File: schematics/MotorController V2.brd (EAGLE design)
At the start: 120.6 x 100 mm, 40 parts, among them IC1 7805, Q1 BC307

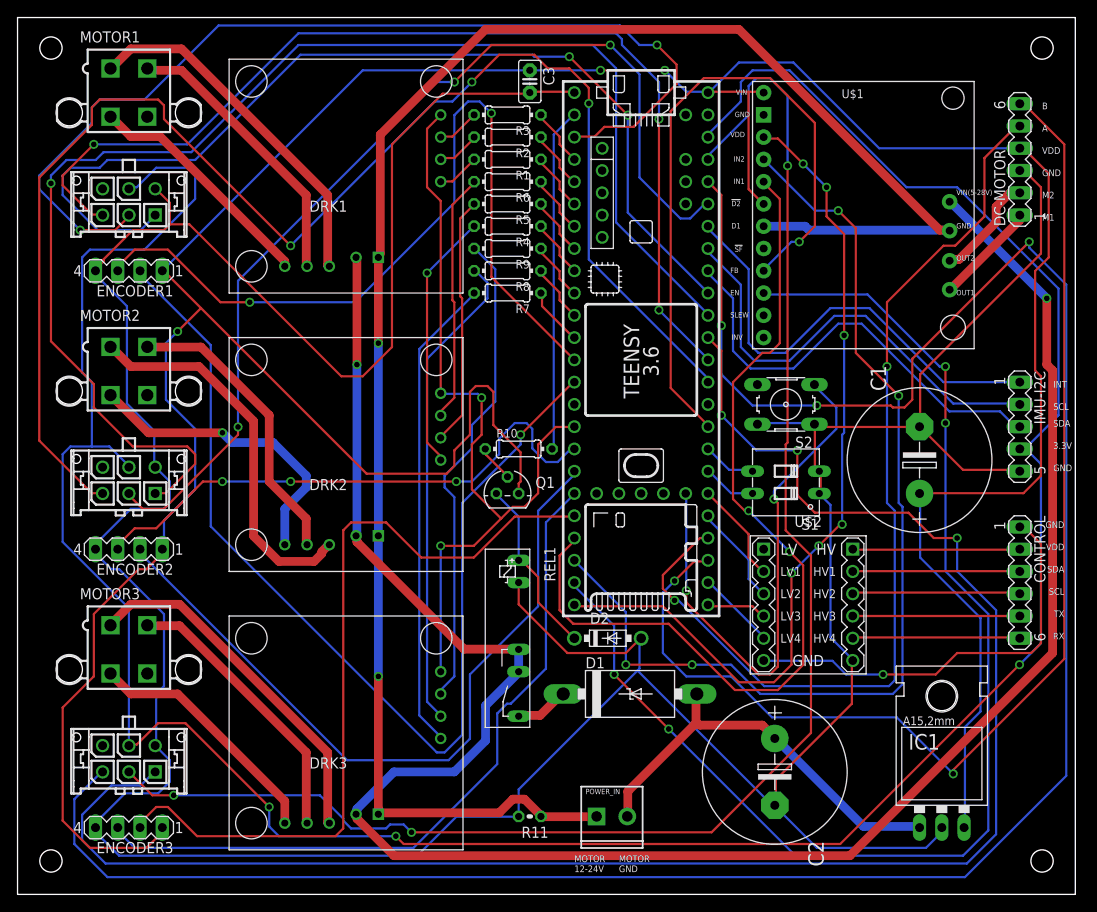
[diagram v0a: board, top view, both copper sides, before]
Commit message: AfterWeekend
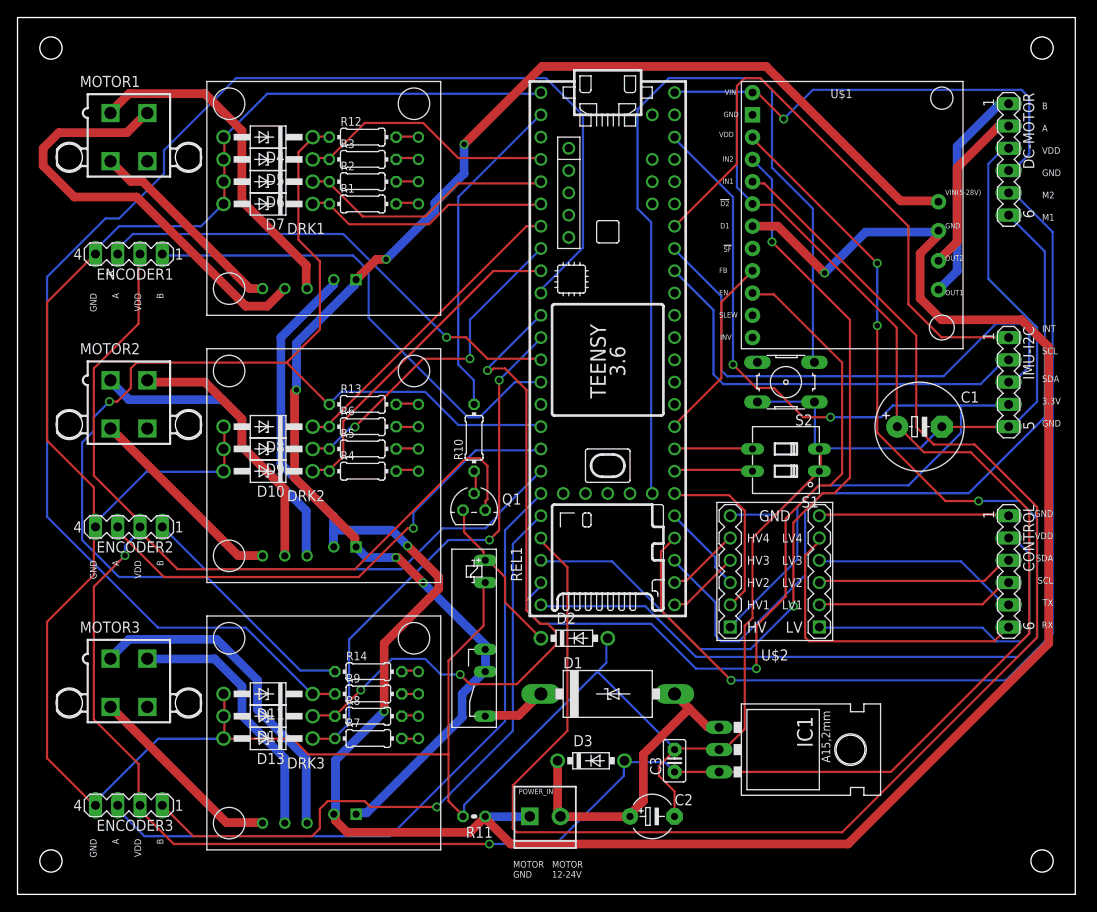
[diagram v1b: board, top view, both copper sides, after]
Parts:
- removed HALL1, HALL2, HALL3: (no value), con-molex-micro-fit-3_0:43045-0612
- added D10, D11, D12, D13, D4, D5, D6, D7, D8, D9: 5.1V, diode:DO41Z10
- added D3: 1N5818-B, diode:DO41-7.6
- added R12, R13, R14: 1K, resistor:0204/7
- C1: value 2200uF -> 1000uF; device rcl:E7,5-16 -> rcl:E5-10,5
- C2: value 2200uF -> 100uF; device rcl:E7,5-16 -> rcl:E5-5
- CONTROL, S1, S2: value (none) -> (none)
- R1, R2, R3: value 330 -> 1K
- moved C3 79.2 mm to (0.00, 1.27), turned to 90 degrees
- moved R7 53.2 mm to (-34.9, 3.81), turned to 0 degrees
- moved R8 53.2 mm to (-34.9, 6.35), turned to 0 degrees
- moved R9 53.2 mm to (-34.9, 8.89), turned to 0 degrees
- moved R6 32.5 mm to (-35.6, 39.4), turned to 0 degrees
- moved R4 32.5 mm to (-35.6, 34.3), turned to 0 degrees
- moved R5 32.5 mm to (-35.6, 36.8), turned to 0 degrees
- moved IC1 22.2 mm to (8.89, 2.54), turned to 270 degrees
- moved R3 17.3 mm to (-35.6, 69.8), turned to 0 degrees
- moved R1 17.3 mm to (-35.6, 64.8), turned to 0 degrees
- moved R2 17.3 mm to (-35.6, 67.3), turned to 0 degrees
- moved C2 14.9 mm to (-2.54, -5.08), turned to 0 degrees
- moved POWER_IN 7.62 mm to (-16.5, -5.08)
- moved R11 6.35 mm to (-22.9, -5.08)
- moved U$2 5.39 mm to (11.4, 22.9), turned to 180 degrees
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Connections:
- net LCTRL-GND renamed CTRL-GND
- net N$48 renamed IMU-INT
- removed net LCTR-RX: CONTROL.6, U$2.HV4
- removed net LCTRL-SCL: CONTROL.4, U$2.HV2
- removed net LCTRL-SDA: CONTROL.3, U$2.HV1
- removed net LCTRL-TX: CONTROL.5, U$2.HV3
- removed net LCTRL-VDD: CONTROL.2, U$2.HV
- removed net LV: U$2.LV
- removed net N$49: HALL3.P$2, PRJ1.23/A9
- removed net N$50: HALL3.P$3, PRJ1.22/A8
- removed net N$51: HALL2.P$2, PRJ1.21/A7
- removed net N$54: HALL1.P$1, PRJ1.17/A3
- removed net N$55: HALL2.P$1, PRJ1.16/A2
- removed net N$56: HALL3.P$1, PRJ1.15/A1
- removed net N$57: HALL1.P$2, PRJ1.1/TX
- removed net N$58: HALL1.P$3, PRJ1.14/A0
- removed net N$59: HALL2.P$3, PRJ1.13/SCK
- new net CTR-SCL: CONTROL.4, U$2.LV1
- new net CTR-SDA: CONTROL.3, U$2.LV2
- new net CTRL-RX: CONTROL.6, U$2.LV4
- new net CTRL-TX: CONTROL.5, U$2.LV3
- new net CTRL-VDD: CONTROL.2, U$2.LV
- new net N$43: DRK1.EN, R12.2
- new net N$46: D4.C, PRJ1.24, R12.1, R13.1, R14.1
- new net N$48: DRK2.EN, R13.2
- net 3.3V: now also U$2.HV; no longer HALL1.P$5, HALL2.P$5, HALL3.P$5
- net GND: now also D10.A, D11.A, D12.A, D13.A, D4.A, D5.A, D6.A, D7.A, D8.A, D9.A; no longer HALL1.P$4, HALL2.P$4, HALL3.P$4
- net IMU-SCL: now also PRJ1.18/A4/SDA; no longer PRJ1.19/A5/SCL
- net IMU-SDA: now also PRJ1.19/A5/SCL; no longer PRJ1.18/A4/SDA
- net N$10: now also R14.2; no longer DRK1.EN, DRK2.EN, PRJ1.24
- net N$21: now also D8.C
- net N$22: now also D9.C
- net N$23: now also D10.C
- net N$27: now also D11.C
- net N$28: now also D12.C
- net N$29: now also D13.C
- net N$32: now also D3.C
- net N$34: now also ENCODER1.1; no longer ENCODER1.2
- net N$36: now also ENCODER2.1; no longer ENCODER2.2
- net N$38: now also ENCODER3.1; no longer ENCODER3.2
- net N$7: now also D7.C
- net N$8: now also D6.C
- net N$9: now also D5.C
- net RX5: now also U$2.HV4; no longer U$2.LV4
- net SCL1: now also U$2.HV1; no longer U$2.LV1
- net SDA1: now also U$2.HV2; no longer U$2.LV2
- net TX5: now also U$2.HV3; no longer U$2.LV3
- net VCC: now also D3.A, ENCODER1.2, ENCODER2.2, ENCODER3.2; no longer ENCODER1.1, ENCODER2.1, ENCODER3.1
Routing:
- net N$50: track 261.6 -> 0.00 mm, vias 3 -> 0
- net 3.3V: track 315.4 -> 105.4 mm, vias 3 -> 2
- net N$56: track 200.8 -> 0.00 mm, vias 3 -> 0
- net N$49: track 175.8 -> 0.00 mm, vias 3 -> 0
- net N$59: track 164.9 -> 0.00 mm, vias 3 -> 0
- net N$27: track 6.68 -> 164.7 mm
- net N$55: track 153.5 -> 0.00 mm, vias 1 -> 0
- net N$46: track 0.00 -> 139.6 mm, vias 0 -> 1
- net N$58: track 118.5 -> 0.00 mm, vias 3 -> 0
- net N$51: track 114.9 -> 0.00 mm, vias 3 -> 0
- net N$57: track 113.5 -> 0.00 mm, vias 2 -> 0
- net N$54: track 112.2 -> 0.00 mm, vias 2 -> 0
- net N$10: track 92.0 -> 2.08 mm, vias 2 -> 0
- net N$28: track 6.70 -> 78.9 mm, vias 0 -> 3
- net N$44: track 103.9 -> 175.1 mm, vias 2 -> 0
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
